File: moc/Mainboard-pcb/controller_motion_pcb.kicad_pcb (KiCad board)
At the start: 4 copper layers, 113 x 54 mm, 24 parts, among them J1 Conn_01x14_Male, J3 Conn_01x15_Male, P0 Conn_01x03, P1 Conn_01x03, P2 Conn_01x03, P3 Conn_01x03, P4 Conn_01x03, P5 Conn_01x03, P6 Conn_01x03, P7 Conn_01x03

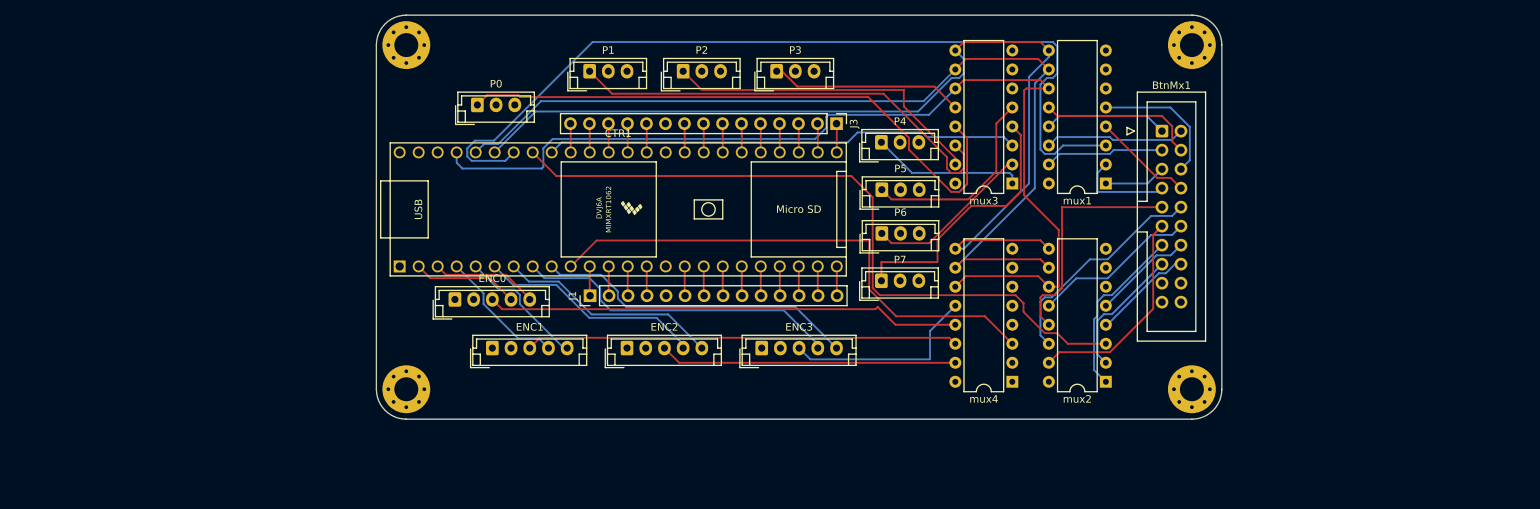
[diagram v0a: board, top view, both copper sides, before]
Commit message: first commit
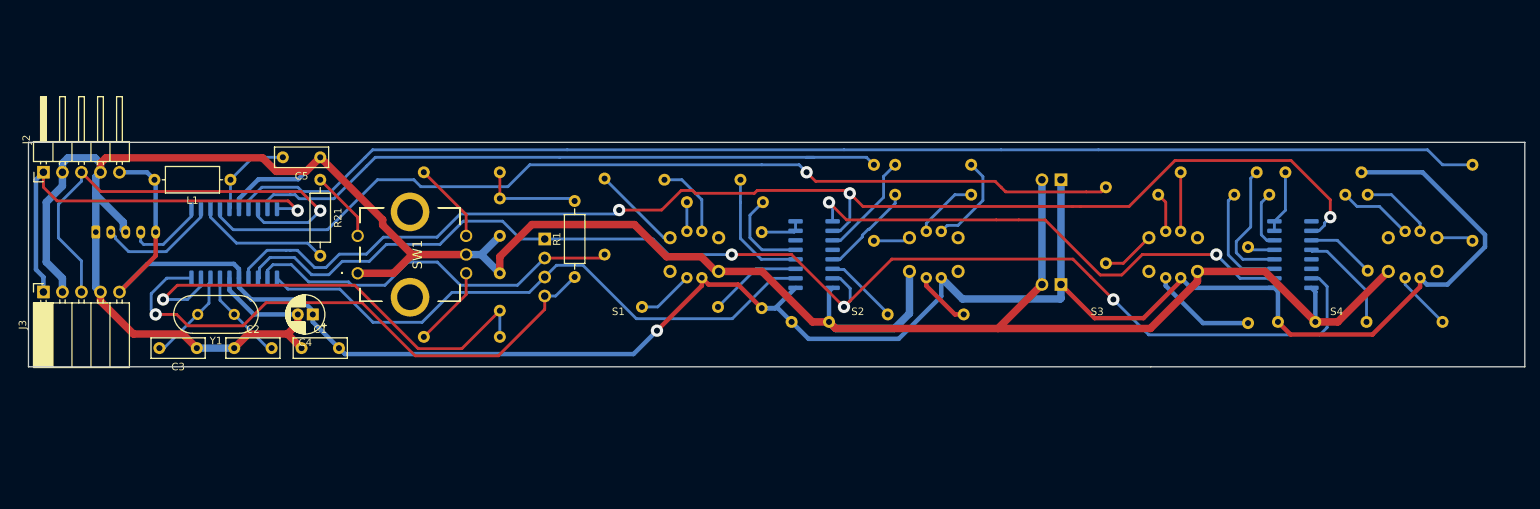
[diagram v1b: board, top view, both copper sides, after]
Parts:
- removed BtnMx1: Conn_02x09_Counter_Clockwise, Connector_IDC:IDC-Header_2x10_P2.54mm_Vertical
- removed CTR1: Teensy4.1, teensy:Teensy41_my
- removed ENC0, ENC1, ENC2, ENC3: Conn_01x05, Connector_JST:JST_EH_B5B-EH-A_1x05_P2.50mm_Vertical
- removed P0, P1, P2, P3, P4, P5, P6, P7: Conn_01x03, Connector_JST:JST_EH_B3B-EH-A_1x03_P2.50mm_Vertical
- removed REF** (x4): MountingHole_3.2mm_M3_Pad_Via, MountingHole:MountingHole_3.2mm_M3_Pad_Via
- removed mux1, mux2, mux3, mux4: 74HC4051, Package_DIP:DIP-16_W7.62mm
- added C1: 100nF, Capacitor_THT:C_Disc_D7.0mm_W2.5mm_P5.00mm, F.Cu at (68.5, 77.5)
- added C2: 22pF, Capacitor_THT:C_Disc_D7.0mm_W2.5mm_P5.00mm, F.Cu at (59.5, 77.5)
- added C3: 22pF, Capacitor_THT:C_Disc_D7.0mm_W2.5mm_P5.00mm, F.Cu at (54.5, 77.5)
- added C4: 10uH, Capacitor_THT:CP_Radial_D5.0mm_P2.00mm, F.Cu at (70.0, 73.0)
- added C5: 100nF, Capacitor_THT:C_Disc_D7.0mm_W2.5mm_P5.00mm, F.Cu at (71.0, 52.0)
- added C6: 100nF, Capacitor_THT:C_Disc_D7.0mm_W2.5mm_P5.00mm, B.Cu at (95.0, 67.5)
- added C7: 100nF, Capacitor_THT:C_Disc_D7.0mm_W2.5mm_P5.00mm, B.Cu at (95.0, 57.5)
- added C8: 100nF, Capacitor_THT:C_Disc_D7.0mm_W2.5mm_P5.00mm, B.Cu at (134.0, 74.0)
- added C9: 100nF, Capacitor_THT:C_Disc_D7.0mm_W2.5mm_P5.00mm, B.Cu at (199.0, 74.0)
- added J2: I2C INTERFACE MSTR, Connector_PinHeader_2.54mm:PinHeader_1x05_P2.54mm_Horizontal, F.Cu at (34.0, 54.0)
- added J4: Conn_01x02_Male, Connector_PinHeader_2.54mm:PinHeader_1x02_P2.54mm_Horizontal, B.Cu at (170.0, 55.0)
- added J5: Conn_01x02_Female, Connector_PinSocket_2.54mm:PinSocket_1x02_P2.54mm_Horizontal, B.Cu at (170.0, 69.0)
- added J6: Conn_01x06_Female, Connector_JST:JST_PH_B5B-PH-K_1x05_P2.00mm_Vertical, B.Cu at (41.0, 62.0)
- added L1: 10uH, Inductor_THT:L_Axial_L7.0mm_D3.3mm_P10.16mm_Horizontal_Fastron_MICC, F.Cu at (59.0, 55.0)
- added R1: 0, Resistor_THT:R_Axial_DIN0207_L6.3mm_D2.5mm_P10.16mm_Horizontal, F.Cu at (105.0, 68.0)
- added R10: 165, Resistor_THT:R_Axial_DIN0207_L6.3mm_D2.5mm_P10.16mm_Horizontal, B.Cu at (158.0, 57.0)
- added R11: 155, Resistor_THT:R_Axial_DIN0207_L6.3mm_D2.5mm_P10.16mm_Horizontal, B.Cu at (158.0, 53.0)
- added R12: 100, Resistor_THT:R_Axial_DIN0207_L6.3mm_D2.5mm_P10.16mm_Horizontal, B.Cu at (157.0, 73.0)
- added R13: 165, Resistor_THT:R_Axial_DIN0207_L6.3mm_D2.5mm_P10.16mm_Horizontal, B.Cu at (183.0, 57.0)
- added R14: 155, Resistor_THT:R_Axial_DIN0207_L6.3mm_D2.5mm_P10.16mm_Horizontal, B.Cu at (186.0, 54.0)
- added R15: 100, Resistor_THT:R_Axial_DIN0207_L6.3mm_D2.5mm_P10.16mm_Horizontal, B.Cu at (195.0, 74.2)
- added R16: 165, Resistor_THT:R_Axial_DIN0207_L6.3mm_D2.5mm_P10.16mm_Horizontal, B.Cu at (208.0, 57.0)
- added R17: 155, Resistor_THT:R_Axial_DIN0207_L6.3mm_D2.5mm_P10.16mm_Horizontal, B.Cu at (211.0, 57.0)
- added R18: 100, Resistor_THT:R_Axial_DIN0207_L6.3mm_D2.5mm_P10.16mm_Horizontal, B.Cu at (221.0, 74.0)
- added R19: 27k, Resistor_THT:R_Axial_DIN0207_L6.3mm_D2.5mm_P10.16mm_Horizontal, B.Cu at (95.0, 76.0)
- added R20: 27k, Resistor_THT:R_Axial_DIN0207_L6.3mm_D2.5mm_P10.16mm_Horizontal, B.Cu at (95.0, 54.0)
- added R21: 4.7k, Resistor_THT:R_Axial_DIN0207_L6.3mm_D2.5mm_P10.16mm_Horizontal, F.Cu at (71.0, 55.0)
- added R22: 10k, Resistor_THT:R_Axial_DIN0207_L6.3mm_D2.5mm_P10.16mm_Horizontal, B.Cu at (130.0, 62.0)
- added R23: 10k, Resistor_THT:R_Axial_DIN0207_L6.3mm_D2.5mm_P10.16mm_Horizontal, B.Cu at (200.0, 54.0)
- added R3: 4.7k, Resistor_THT:R_Axial_DIN0207_L6.3mm_D2.5mm_P10.16mm_Horizontal, B.Cu at (109.0, 65.0)
- added R4: 4.7k, Resistor_THT:R_Axial_DIN0207_L6.3mm_D2.5mm_P10.16mm_Horizontal, B.Cu at (145.0, 53.0)
- added R5: 4.7k, Resistor_THT:R_Axial_DIN0207_L6.3mm_D2.5mm_P10.16mm_Horizontal, B.Cu at (176.0, 56.0)
- added R6: 4.7k, Resistor_THT:R_Axial_DIN0207_L6.3mm_D2.5mm_P10.16mm_Horizontal, B.Cu at (225.0, 53.0)
- added R7: 165, Resistor_THT:R_Axial_DIN0207_L6.3mm_D2.5mm_P10.16mm_Horizontal, B.Cu at (120.0, 58.0)
- added R8: 155, Resistor_THT:R_Axial_DIN0207_L6.3mm_D2.5mm_P10.16mm_Horizontal, B.Cu at (117.0, 55.0)
- added R9: 100, Resistor_THT:R_Axial_DIN0207_L6.3mm_D2.5mm_P10.16mm_Horizontal, B.Cu at (114.0, 72.0)
- added S1: 228CMVARGBFR, flex-Ambisonic:228CMVARGBFR, F.Cu at (121.0, 65.0)
- added S2: 228CMVARGBFR, flex-Ambisonic:228CMVARGBFR, F.Cu at (153.0, 65.0)
- added S3: 228CMVARGBFR, flex-Ambisonic:228CMVARGBFR, F.Cu at (185.0, 65.0)
- added S4: 228CMVARGBFR, flex-Ambisonic:228CMVARGBFR, F.Cu at (217.0, 65.0)
- added SW1: Rotary_Encoder_Switch, MOUSERfootprintANDsymbol:PEC11R4230KS0024, F.Cu at (83.0, 67.5)
- added U1: ATtiny861V-10SU, Package_SO:SOIC-20W_7.5x12.8mm_P1.27mm, B.Cu at (59.5, 63.5)
- added U2: TPIC6C595-SOIC, Package_SO:SOIC-16_3.9x9.9mm_P1.27mm, B.Cu at (137.0, 65.0)
- added U3: TPIC6C595-SOIC, Package_SO:SOIC-16_3.9x9.9mm_P1.27mm, B.Cu at (201.0, 65.0)
- added Y1: Crystal, Crystal:Crystal_HC49-U_Vertical, F.Cu at (59.5, 73.0)
- J1: value Conn_01x14_Male -> ICSP INTERFACE; footprint Connector_PinHeader_2.54mm:PinHeader_1x14_P2.54mm_Vertical -> Connector_PinHeader_2.54mm:PinHeader_1x04_P2.54mm_Vertical; moved to B.Cu
- J3: value Conn_01x15_Male -> I2C INTERFACE SLAV; footprint Connector_PinHeader_2.54mm:PinHeader_1x15_P2.54mm_Vertical -> Connector_PinSocket_2.54mm:PinSocket_1x05_P2.54mm_Horizontal
- moved J3 108.4 mm to (34.0, 70.0), turned to 90 degrees
- moved J1 9.70 mm to (101.0, 62.9), turned to 180 degrees
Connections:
- J1 pad 1: Net-(CTR1-Pad11) -> PSHFCLK
- J1 pad 2: Net-(CTR1-Pad12) -> MISO
- J1 pad 3: Net-(CTR1-Pad13) -> MOSI
- J1 pad 4: Net-(CTR1-Pad14) -> RESET
- J3 pad 1: Net-(CTR1-Pad25) -> SDA
- J3 pad 2: Net-(CTR1-Pad26) -> GND
- J3 pad 3: Net-(CTR1-Pad27) -> SCL
- J3 pad 4: Net-(CTR1-Pad28) -> GND
- J3 pad 5: Net-(CTR1-Pad29) -> ATM_VCC
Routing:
- net GND: track 0.00 -> 374.3 mm
- net ATM_VCC: track 0.00 -> 287.1 mm, vias 0 -> 1
- net PSHFCLK: track 0.00 -> 174.5 mm, vias 0 -> 3
- net PSHFUDATE: track 0.00 -> 170.5 mm, vias 0 -> 3
- net PB3: track 0.00 -> 168.8 mm
- net s0: track 135.1 -> 0.00 mm
- net s2: track 129.8 -> 0.00 mm
- net s1: track 127.5 -> 0.00 mm
- net PB2: track 0.00 -> 126.3 mm, vias 0 -> 1
- net mux_btnMx1: track 117.6 -> 0.00 mm
- net mux_btnMx2: track 95.4 -> 0.00 mm
- net PB1: track 0.00 -> 86.4 mm
- net Net-(P0-Pad1): track 81.1 -> 0.00 mm
- net MOSI: track 0.00 -> 80.1 mm
- net RESET: track 0.00 -> 75.5 mm, vias 0 -> 1
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- removed copper zone on In2.Cu, net +3V3
- removed copper zone on In1.Cu, net GND
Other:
- board size 113 x 54 mm -> 200 x 30 mm
- copper layers 4 -> 2
- net class Default: clearance 0.2 -> 0.4; trace_width 0.25 -> 0.381; via_dia 0.8 -> 1.65; via_drill 0.4 -> 0.8
- net class VCC added: clearance 0.4, trace_width 0.6, via_dia 1.65, via_drill 0.8
- rule trace_clearance: 0.2 -> 0.4
- board text removed: "AAA Motion_Ctr-0.001"

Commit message: MCU and Controller board done
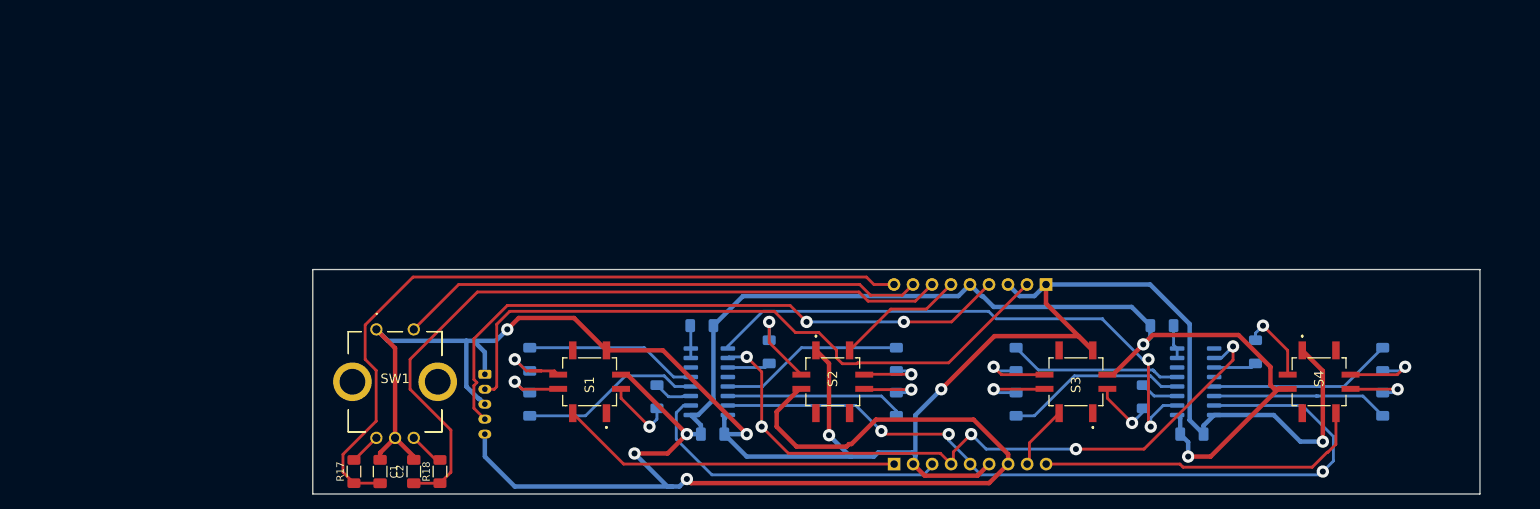
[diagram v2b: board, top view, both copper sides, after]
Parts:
- removed C5, C6, C7, C8, C9: 100nF, Capacitor_THT:C_Disc_D7.0mm_W2.5mm_P5.00mm
- removed J4: Conn_01x02_Male, Connector_PinHeader_2.54mm:PinHeader_1x02_P2.54mm_Horizontal
- removed J5: Conn_01x02_Female, Connector_PinSocket_2.54mm:PinSocket_1x02_P2.54mm_Horizontal
- removed J6: Conn_01x06_Female, Connector_JST:JST_PH_B5B-PH-K_1x05_P2.00mm_Vertical
- removed L1: 10uH, Inductor_THT:L_Axial_L7.0mm_D3.3mm_P10.16mm_Horizontal_Fastron_MICC
- removed R1: 0, Resistor_THT:R_Axial_DIN0207_L6.3mm_D2.5mm_P10.16mm_Horizontal
- removed R19: 27k, Resistor_THT:R_Axial_DIN0207_L6.3mm_D2.5mm_P10.16mm_Horizontal
- removed R22, R23: 10k, Resistor_THT:R_Axial_DIN0207_L6.3mm_D2.5mm_P10.16mm_Horizontal
- removed R3, R4: 4.7k, Resistor_THT:R_Axial_DIN0207_L6.3mm_D2.5mm_P10.16mm_Horizontal
- removed U3: TPIC6C595-SOIC, Package_SO:SOIC-16_3.9x9.9mm_P1.27mm
- removed Y1: Crystal, Crystal:Crystal_HC49-U_Vertical
- C1: footprint Capacitor_THT:C_Disc_D7.0mm_W2.5mm_P5.00mm -> Capacitor_SMD:C_1206_3216Metric_Pad1.33x1.80mm_HandSolder
- C2: value 22pF -> 100nF; footprint Capacitor_THT:C_Disc_D7.0mm_W2.5mm_P5.00mm -> Capacitor_SMD:C_1206_3216Metric_Pad1.33x1.80mm_HandSolder
- C3: value 22pF -> 100nF; footprint Capacitor_THT:C_Disc_D7.0mm_W2.5mm_P5.00mm -> Capacitor_SMD:C_1206_3216Metric_Pad1.33x1.80mm_HandSolder; moved to B.Cu
- C4: value 10uH -> 100nF; footprint Capacitor_THT:CP_Radial_D5.0mm_P2.00mm -> Capacitor_SMD:C_1206_3216Metric_Pad1.33x1.80mm_HandSolder; moved to B.Cu
- J1: value ICSP INTERFACE -> Conn_01x09_Male; footprint Connector_PinHeader_2.54mm:PinHeader_1x04_P2.54mm_Vertical -> Connector_PinHeader_2.54mm:PinHeader_1x09_P2.54mm_Vertical
- J2: value I2C INTERFACE MSTR -> Conn_01x09_Male; footprint Connector_PinHeader_2.54mm:PinHeader_1x05_P2.54mm_Horizontal -> Connector_PinHeader_2.54mm:PinHeader_1x09_P2.54mm_Vertical; moved to B.Cu
- J3: value I2C INTERFACE SLAV -> Conn_01x06_Female; footprint Connector_PinSocket_2.54mm:PinSocket_1x05_P2.54mm_Horizontal -> Connector_JST:JST_PH_B5B-PH-K_1x05_P2.00mm_Vertical; moved to B.Cu
- R10, R13, R16, R7: value 165 -> 100; footprint Resistor_THT:R_Axial_DIN0207_L6.3mm_D2.5mm_P10.16mm_Horizontal -> Resistor_SMD:R_1206_3216Metric_Pad1.30x1.75mm_HandSolder
- R11, R14, R8: value 155 -> 165; footprint Resistor_THT:R_Axial_DIN0207_L6.3mm_D2.5mm_P10.16mm_Horizontal -> Resistor_SMD:R_1206_3216Metric_Pad1.30x1.75mm_HandSolder
- R12, R15, R9: value 100 -> 155; footprint Resistor_THT:R_Axial_DIN0207_L6.3mm_D2.5mm_P10.16mm_Horizontal -> Resistor_SMD:R_1206_3216Metric_Pad1.30x1.75mm_HandSolder
- R17: value 155 -> 27k; footprint Resistor_THT:R_Axial_DIN0207_L6.3mm_D2.5mm_P10.16mm_Horizontal -> Resistor_SMD:R_1206_3216Metric_Pad1.30x1.75mm_HandSolder; moved to F.Cu
- R18: value 100 -> 27k; footprint Resistor_THT:R_Axial_DIN0207_L6.3mm_D2.5mm_P10.16mm_Horizontal -> Resistor_SMD:R_1206_3216Metric_Pad1.30x1.75mm_HandSolder; moved to F.Cu
- R20: value 27k -> 10k; footprint Resistor_THT:R_Axial_DIN0207_L6.3mm_D2.5mm_P10.16mm_Horizontal -> Resistor_SMD:R_1206_3216Metric_Pad1.30x1.75mm_HandSolder
- R21: value 4.7k -> 10k; footprint Resistor_THT:R_Axial_DIN0207_L6.3mm_D2.5mm_P10.16mm_Horizontal -> Resistor_SMD:R_1206_3216Metric_Pad1.30x1.75mm_HandSolder; moved to B.Cu
- R5: value 4.7k -> 165; footprint Resistor_THT:R_Axial_DIN0207_L6.3mm_D2.5mm_P10.16mm_Horizontal -> Resistor_SMD:R_1206_3216Metric_Pad1.30x1.75mm_HandSolder
- R6: value 4.7k -> 155; footprint Resistor_THT:R_Axial_DIN0207_L6.3mm_D2.5mm_P10.16mm_Horizontal -> Resistor_SMD:R_1206_3216Metric_Pad1.30x1.75mm_HandSolder
- S1, S2, S3, S4: footprint flex-Ambisonic:228CMVARGBFR -> MOUSERfootprintANDsymbol:228CMVARGBFR
- U1: value ATtiny861V-10SU -> TPIC6C595-SOIC; footprint Package_SO:SOIC-20W_7.5x12.8mm_P1.27mm -> Package_SO:SOIC-16_3.9x9.9mm_P1.27mm
- moved R17 140.5 mm to (75.5, 94.0), turned to 90 degrees
- moved R18 135.5 mm to (87.0, 94.0), turned to 90 degrees
- moved R6 128.7 mm to (99.0, 79.0), turned to 90 degrees
- moved J2 120.2 mm to (147.7, 93.0), turned to 270 degrees
- moved C4 118.6 mm to (187.5, 89.0), turned to 0 degrees
- moved R21 114.2 mm to (183.5, 74.5), turned to 180 degrees
- moved R5 82.3 mm to (99.0, 85.0)
- moved C3 69.9 mm to (123.4, 89.0), turned to 0 degrees
- moved J1 67.3 mm to (168.0, 69.0), turned to 90 degrees
- moved U1 66.1 mm to (123.0, 82.0), turned to 0 degrees
- moved J3 60.0 mm to (93.0, 81.0), turned to 270 degrees
- moved U2 53.8 mm to (188.0, 82.0)
- moved R8 39.2 mm to (148.0, 79.0), turned to 90 degrees
- moved R14 36.8 mm to (213.0, 79.0), turned to 90 degrees
- moved R9 36.4 mm to (148.0, 85.0), turned to 270 degrees
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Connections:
- C1 pad 2: ATM_VCC -> ENCA
- C2 pad 1: GND -> ENCB
- C2 pad 2: XTAL1 -> GND
- C3 pad 1: GND -> VCC
- C3 pad 2: XTAL2 -> GND
- C4 pad 1: ATM_VCC -> VCC
- J1 pad 1: PSHFCLK -> GND
- J1 pad 2: MISO -> ADC1
- J1 pad 3: MOSI -> GND
- J1 pad 4: RESET -> ADC0
- J2 pad 1: SDA -> PB0
- J2 pad 3: SCL -> PSHFDATA
- J2 pad 4: GND -> PSHFUDATE
- J2 pad 5: ATM_VCC -> PSHFCLK
- J3 pad 1: SDA -> GND
- J3 pad 2: GND -> ADC1
- J3 pad 3: SCL -> GND
- J3 pad 4: GND -> ADC0
- J3 pad 5: ATM_VCC -> VCC
- R10 pad 2: S2_R -> S2_B
- R11 pad 2: Net-(R11-Pad2) -> S3_R
- R12 pad 2: Net-(R12-Pad2) -> S3_G
- R13 pad 2: Net-(R13-Pad2) -> S3_B
- R14 pad 2: Net-(R14-Pad2) -> S4_R
- R15 pad 2: Net-(R15-Pad2) -> S4_G
- R16 pad 2: Net-(R16-Pad2) -> S4_B
- R17 pad 1: Net-(R17-Pad1) -> ENCA
- R18 pad 1: Net-(R18-Pad1) -> ENCB
- R20 pad 1: ENCB -> Net-(R20-Pad1)
- R20 pad 2: Net-(R20-Pad2) -> VCC
- R21 pad 2: ENCSW -> VCC
- R5 pad 1: PB2 -> Net-(R5-Pad1)
- R5 pad 2: Net-(R5-Pad2) -> S1_R
- R6 pad 1: PB3 -> Net-(R6-Pad1)
- R6 pad 2: Net-(R6-Pad2) -> S1_G
- R7 pad 2: S1_R -> S1_b
- R8 pad 2: S1_G -> S2_R
- R9 pad 2: S1_b -> S2_G
- S1 pad 3: Net-(R3-Pad2) -> PB0
- S1 pad 5: Net-(R9-Pad1) -> Net-(R7-Pad1)
- S1 pad 6: Net-(R7-Pad1) -> Net-(R5-Pad1)
- S1 pad 7: ATM_VCC -> VCC
- S1 pad 8: Net-(R8-Pad1) -> Net-(R6-Pad1)
- S2 pad 3: Net-(R4-Pad2) -> PB1
- S2 pad 5: Net-(R12-Pad1) -> Net-(R10-Pad1)
- S2 pad 6: Net-(R10-Pad1) -> Net-(R8-Pad1)
- S2 pad 7: ATM_VCC -> VCC
- S2 pad 8: Net-(R11-Pad1) -> Net-(R9-Pad1)
- S3 pad 3: Net-(R5-Pad2) -> PB2
- S3 pad 5: Net-(R15-Pad1) -> Net-(R13-Pad1)
- S3 pad 6: Net-(R13-Pad1) -> Net-(R11-Pad1)
- S3 pad 7: ATM_VCC -> VCC
- S3 pad 8: Net-(R14-Pad1) -> Net-(R12-Pad1)
- S4 pad 4: Net-(R6-Pad2) -> PB3
- S4 pad 5: Net-(R18-Pad1) -> Net-(R16-Pad1)
- S4 pad 6: Net-(R16-Pad1) -> Net-(R14-Pad1)
- S4 pad 7: ATM_VCC -> VCC
- S4 pad 8: Net-(R17-Pad1) -> Net-(R15-Pad1)
- SW1 pad A: Net-(R19-Pad2) -> Net-(R17-Pad2)
- SW1 pad B: Net-(R20-Pad2) -> Net-(R18-Pad2)
- SW1 pad S2: Net-(R21-Pad1) -> ENCSW
- U1 pad 1: MOSI -> VCC
- U1 pad 10: RESET -> PSHFUDATE
- U1 pad 11: ADC0 -> S2_B
- U1 pad 12: ADC1 -> (no net)
- U1 pad 13: ENCSW -> S2_R
- U1 pad 14: PB2 -> S2_G
- U1 pad 15: Net-(C5-Pad2) -> PSHFCLK
- U1 pad 2: MISO -> PSHFDATA
- U1 pad 3: PSHFCLK -> S1_b
- U1 pad 4: PSHFUDATE -> S1_R
- U1 pad 5: ATM_VCC -> S1_G
- U1 pad 6: GND -> (no net)
- U1 pad 7: XTAL1 -> Net-(R20-Pad1)
- U1 pad 8: XTAL2 -> Net-(R20-Pad1)
- U1 pad 9: ENCA -> Net-(U1-Pad9)
- U2 pad 1: ATM_VCC -> VCC
- U2 pad 11: Net-(R11-Pad2) -> S4_B
- U2 pad 13: S2_R -> S4_R
- U2 pad 14: Net-(R12-Pad2) -> S4_G
- U2 pad 2: MOSI -> Net-(U1-Pad9)
- U2 pad 3: S1_b -> S3_B
- U2 pad 4: S1_G -> S3_R
- U2 pad 5: S1_R -> S3_G
- U2 pad 7: Net-(R22-Pad1) -> Net-(R21-Pad1)
- U2 pad 8: Net-(R22-Pad1) -> Net-(R21-Pad1)
- U2 pad 9: Net-(U2-Pad9) -> (no net)
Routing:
- net ATM_VCC: track 287.1 -> 0.00 mm, vias 1 -> 0
- net VCC: track 0.00 -> 285.7 mm, vias 0 -> 5
- net PB3: track 168.8 -> 44.0 mm
- net PB2: track 126.3 -> 8.44 mm, vias 1 -> 0
- net GND: track 374.3 -> 278.9 mm, vias 0 -> 5
- net ENCB: track 13.6 -> 97.8 mm
- net MOSI: track 80.1 -> 0.00 mm
- net PSHFUDATE: track 170.5 -> 90.9 mm, vias 3 -> 5
- net Net-(U1-Pad9): track 0.00 -> 75.7 mm, vias 0 -> 2
- net RESET: track 75.5 -> 0.00 mm, vias 1 -> 0
- net ADC0: track 10.8 -> 85.4 mm, vias 0 -> 2
- net ADC1: track 16.3 -> 89.6 mm
- net PB1: track 86.4 -> 17.2 mm
- net Net-(U2-Pad9): track 68.7 -> 0.00 mm, vias 2 -> 0
- net PSHFCLK: track 174.5 -> 107.9 mm
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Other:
- board size 200 x 30 mm -> 156 x 30 mm
